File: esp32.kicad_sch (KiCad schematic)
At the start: 32 parts, among them U12 ESP-PSRAM32, U26 SRV05-4, U4 W25Q128, U5 ESP32-S3, Y1 40MHz

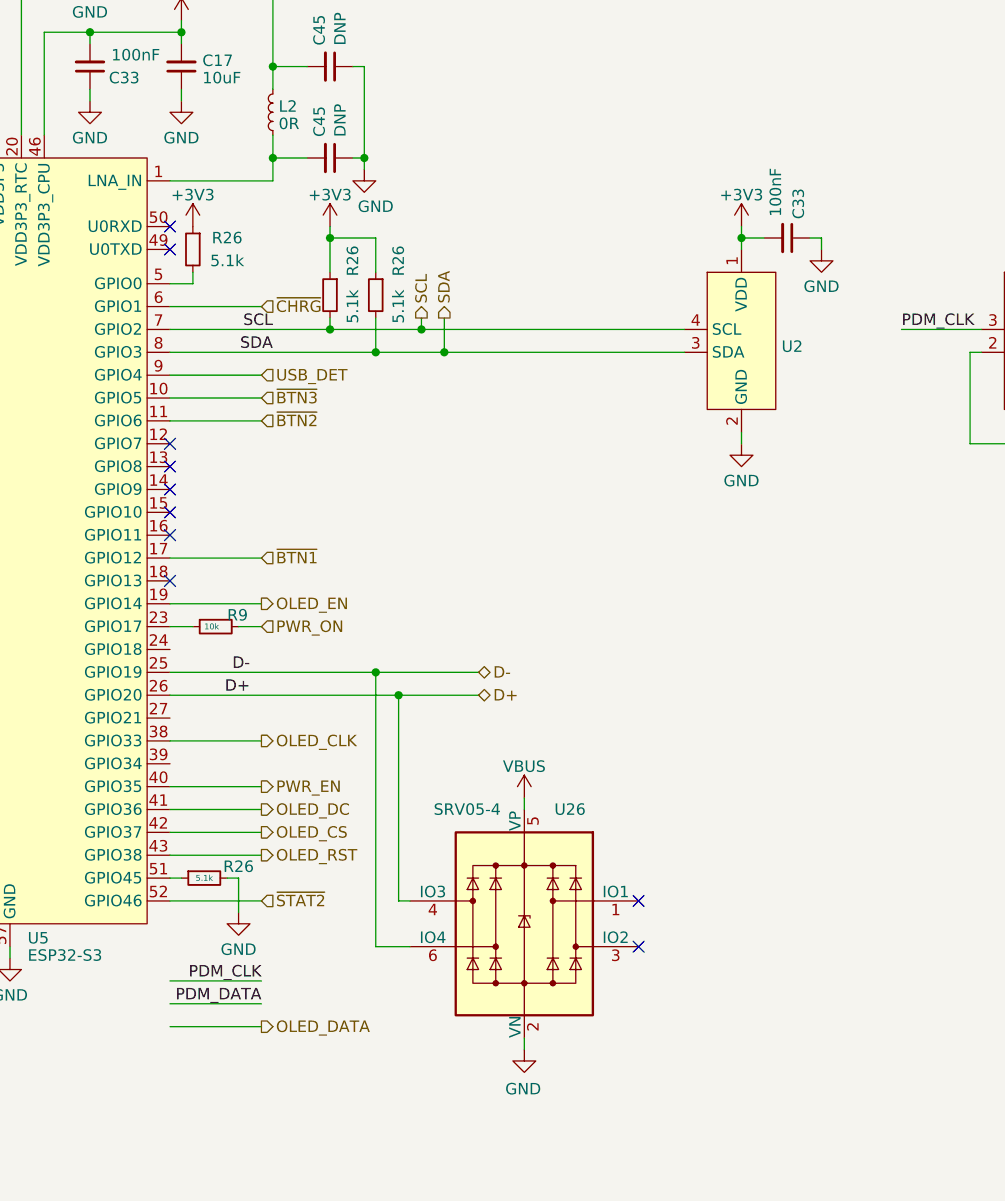
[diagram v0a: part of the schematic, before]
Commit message: Finsh first layout iteration
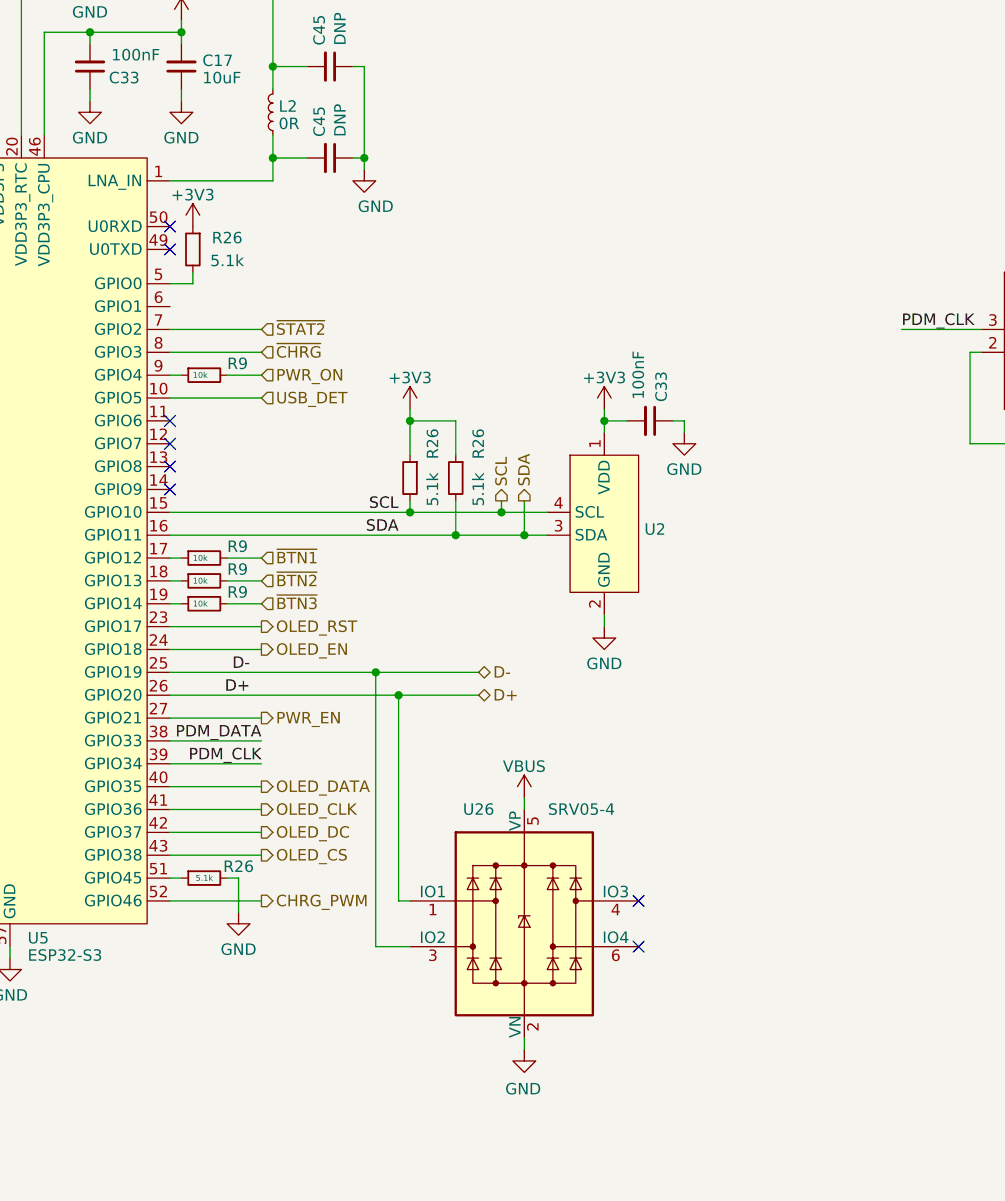
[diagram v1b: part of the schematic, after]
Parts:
- added R9 (x3): 10k, Resistor_SMD:R_0402_1005Metric, symbol Device:R_Small
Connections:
- net D+: now also U26.1 (IO1); no longer U26.4 (IO3)
- net D-: now also U26.3 (IO2); no longer U26.6 (IO4)
- net OLED_CLK: now also U5.41 (GPIO36); no longer U5.38 (GPIO33)
- net OLED_CS: now also U5.43 (GPIO38); no longer U5.42 (GPIO37)
- net OLED_DATA: now also U5.40 (GPIO35)
- net OLED_DC: now also U5.42 (GPIO37); no longer U5.41 (GPIO36)
- net OLED_EN: now also U5.24 (GPIO18); no longer U5.19 (GPIO14)
- net OLED_RST: now also U5.23 (GPIO17); no longer U5.43 (GPIO38)
- net PDM_CLK: now also U5.39 (GPIO34)
- net PDM_DATA: now also U5.38 (GPIO33)
- net PWR_EN: now also U5.27 (GPIO21); no longer U5.40 (GPIO35)
- net SCL: now also U5.15 (GPIO10); no longer U5.7 (GPIO2)
- net SDA: now also U5.16 (GPIO11); no longer U5.8 (GPIO3)
- net USB_DET: now also U5.10 (GPIO5); no longer U5.9 (GPIO4)
- net ~{BTN1}: now also R9.2; no longer U5.17 (GPIO12)
- net ~{BTN2}: now also R9.2; no longer U5.11 (GPIO6)
- net ~{BTN3}: now also R9.2; no longer U5.10 (GPIO5)
- net ~{CHRG}: now also U5.8 (GPIO3); no longer U5.6 (GPIO1)
- net ~{STAT2}: now also U5.7 (GPIO2); no longer U5.52 (GPIO46)
- net at R9.1: now also U5.9 (GPIO4); no longer U5.23 (GPIO17)
- net at U5.18 (GPIO13): now also R9.1
- new net: R9.1, U5.19 (GPIO14)
- new net: R9.1, U5.17 (GPIO12)
- new net CHRG_PWM: U5.52 (GPIO46)
- no-connect marks 18 -> 16
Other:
- moved on the sheet: C33, R26, R9, U2

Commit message: Replace microphone by one from another manufacturer
Previous ones were often DOA.
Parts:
- U3: LCSC C966942 -> C2937733
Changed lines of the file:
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@@
       (effects (font (size 1.27 1.27)) hide)
     )
-    (property "LCSC" "C966942" (at 201.93 86.36 0)
+    (property "LCSC" "C2937733" (at 201.93 86.36 0)
       (effects (font (size 1.27 1.27)) hide)
     )
